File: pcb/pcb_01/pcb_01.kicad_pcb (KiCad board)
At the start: 2 copper layers, 45.7 x 45.7 mm, 6 parts, among them J1 Screw_Terminal_01x02, J2 Screw_Terminal_01x03, J3 Screw_Terminal_01x02, U1 LM358

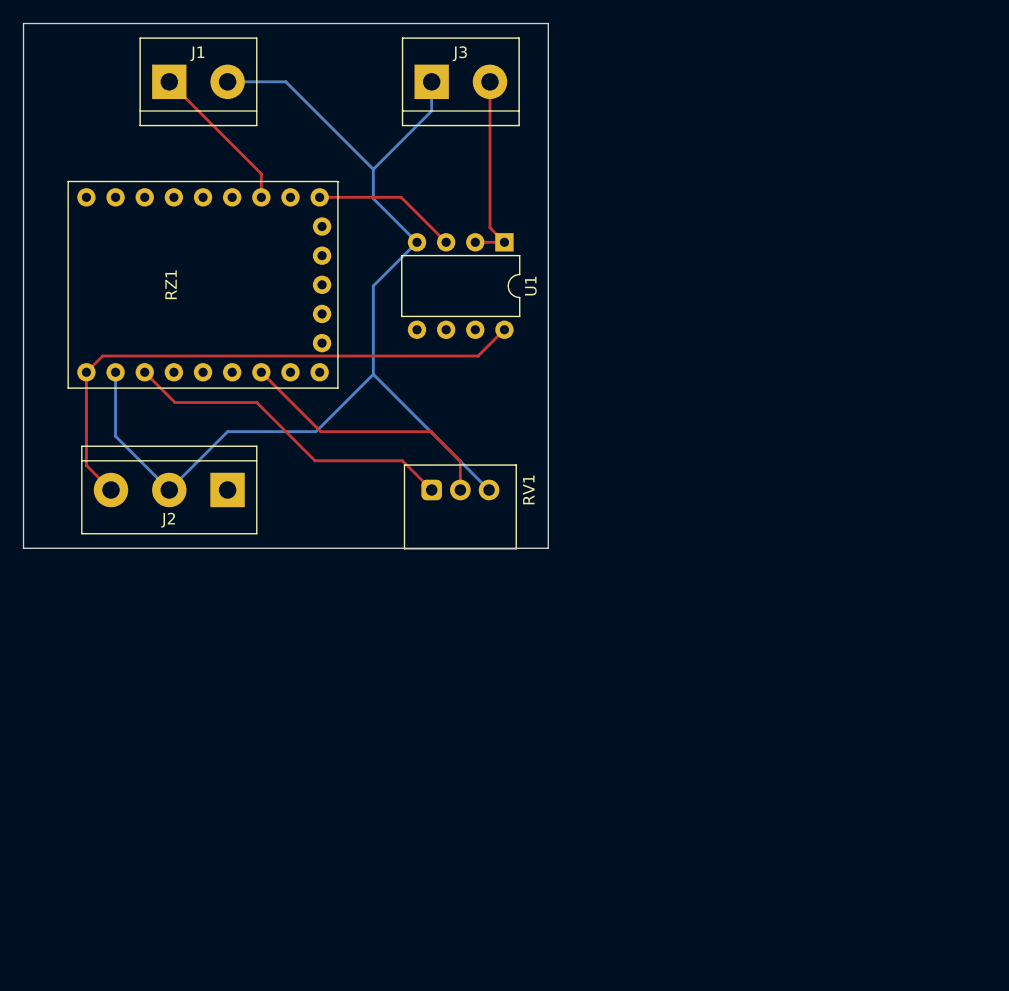
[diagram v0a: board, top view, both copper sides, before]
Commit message: update pcb
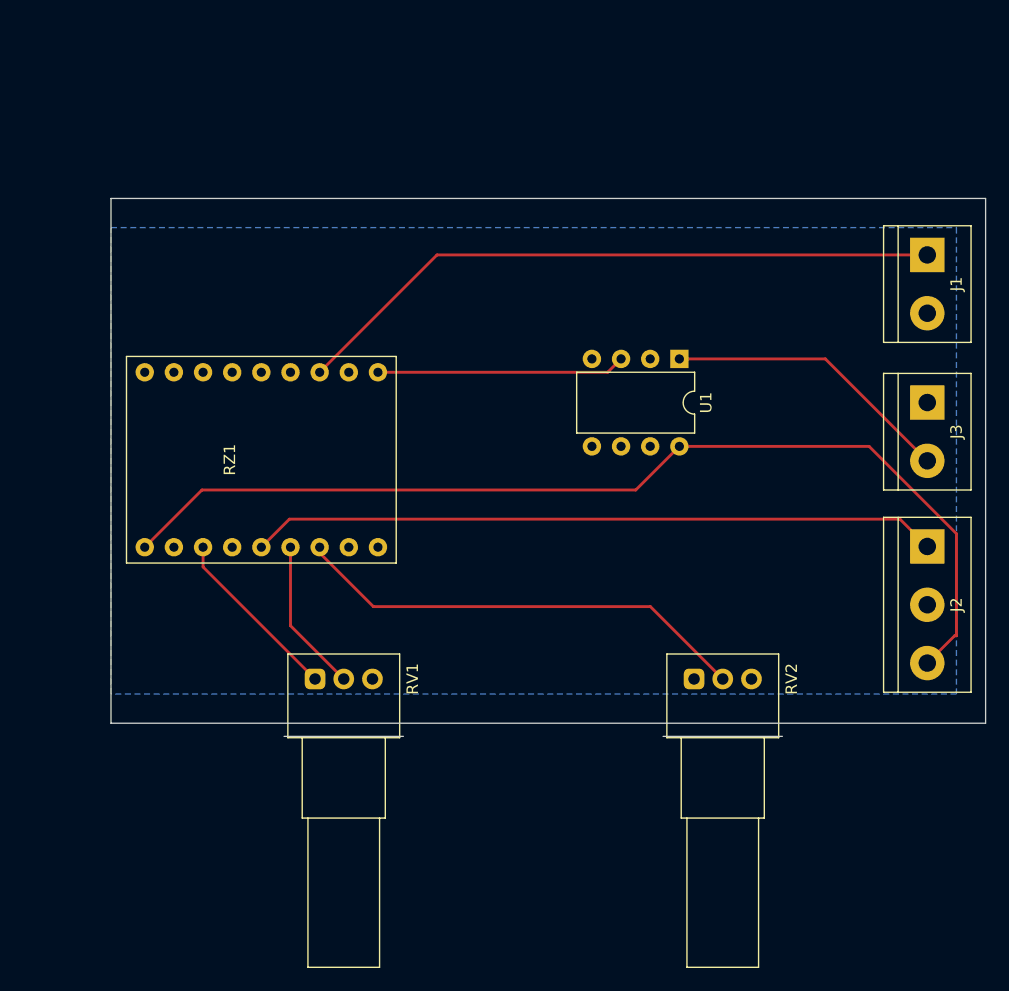
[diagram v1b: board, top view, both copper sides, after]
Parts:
- added RV2: R_Potentiometer, Potentiometer_THT:Potentiometer_Alps_RK097_Single_Horizontal, F.Cu at (167.6, 128.2)
- RZ1: value RP2040-Zero -> RP2040-Zero_1; footprint rp2040-zero:RP2040-Zero -> rp2040-zero:RP2040-Zero_copia
- moved J1 67.7 mm to (188.0, 91.3), turned to -90 degrees
- moved J2 61.2 mm to (188.0, 116.7), turned to -90 degrees
- moved J3 51.4 mm to (188.0, 104.1), turned to -90 degrees
- moved RV1 19.3 mm to (134.6, 128.2)
- moved U1 18.3 mm to (166.4, 100.3)
- moved RZ1 16.1 mm to (141.7, 118.1)
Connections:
- net Net-(J1-Pad2) renamed Earth
- J2 pad 1: Net-(J2-Pad1) -> Net-(RZ1-Pad19)
- RZ1 pad 17: Net-(RV1-Pad2) -> Net-(RZ1-Pad17)
- RZ1 pad 18: Net-(J2-Pad1) -> Net-(RV1-Pad2)
- RZ1 pad 19: unconnected-(RZ1-Pad19) -> Net-(RZ1-Pad19)
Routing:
- net Earth: track 95.0 -> 0.00 mm
- net Net-(RZ1-Pad19): track 0.00 -> 60.0 mm
- net Net-(J1-Pad1): track 13.4 -> 57.2 mm
- net Net-(J2-Pad3): track 49.1 -> 89.9 mm
- net Net-(RZ1-Pad17): track 0.00 -> 40.2 mm
- net Net-(RV1-Pad1): track 29.2 -> 15.5 mm
- net Net-(RV1-Pad2): track 23.1 -> 13.4 mm
- net Net-(U1-Pad3): track 12.6 -> 21.7 mm
- net Net-(J3-Pad2): track 17.0 -> 25.3 mm
- net Net-(J2-Pad1): track 0.57 -> 0.00 mm
- added copper zone on B.Cu, net Earth
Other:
- board size 45.7 x 45.7 mm -> 76.2 x 45.7 mm

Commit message: update pcb
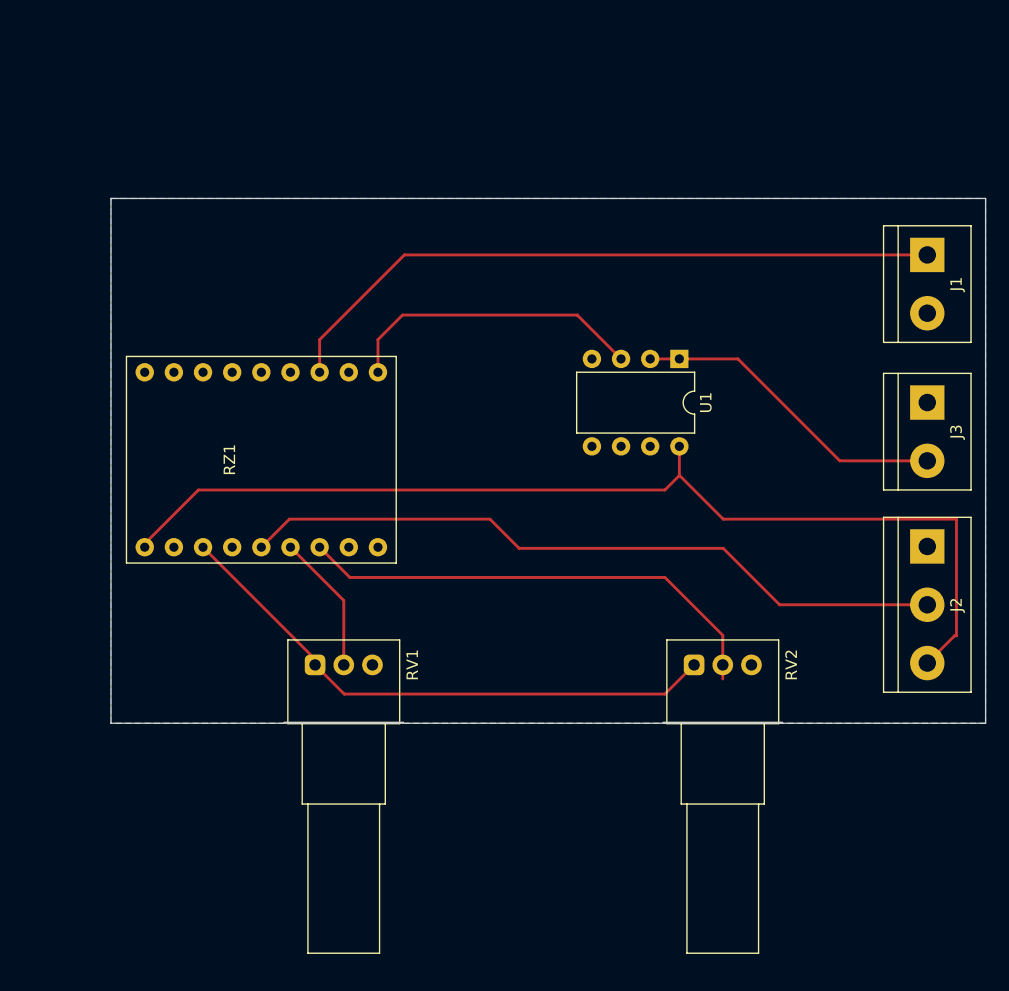
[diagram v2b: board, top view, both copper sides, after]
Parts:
- moved RV1 1.22 mm to (134.6, 127.0)
- moved RV2 1.22 mm to (167.6, 127.0)
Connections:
- J2 pad 1: Net-(RZ1-Pad19) -> Earth
- J2 pad 2: Earth -> Net-(RZ1-Pad19)
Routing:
- net Net-(RV1-Pad1): track 15.5 -> 49.4 mm
- net Net-(RZ1-Pad9): track 21.7 -> 26.5 mm
- net Net-(J3-Pad2): track 25.3 -> 27.8 mm
- net Net-(RZ1-Pad19): track 60.0 -> 62.1 mm
- net Net-(RV2-Pad2): track 40.2 -> 42.1 mm
- net Net-(J1-Pad1): track 57.2 -> 58.8 mm
- net Net-(J2-Pad3): track 89.9 -> 91.5 mm
- net Net-(RV1-Pad2): track 13.4 -> 12.2 mm
